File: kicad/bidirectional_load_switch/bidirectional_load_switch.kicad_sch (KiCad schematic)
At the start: 30 parts, among them J101 1017503, J102 Conn_01x02_Socket, J103 Conn_01x09_Socket, J104 Conn_01x02_Socket, J105 Conn_01x02_Socket, J106 Conn_01x02_Socket, J107 AVR-ISP-6, SW101 PTS526 SK15 SMTR2 LFS, U101 TMCS1101A3BQDRQ1, U102 TLV75733PDBVR, U103 ATTINY85-20SU

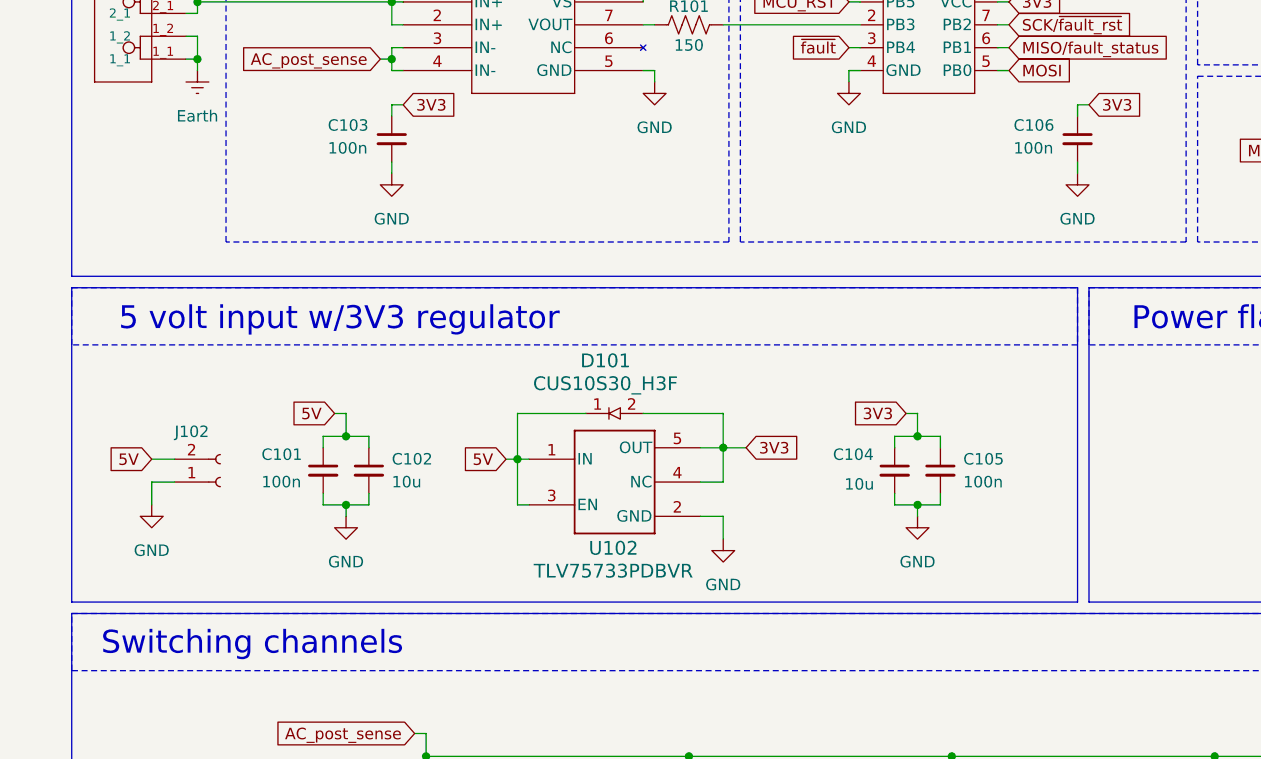
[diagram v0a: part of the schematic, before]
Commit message: ready for order
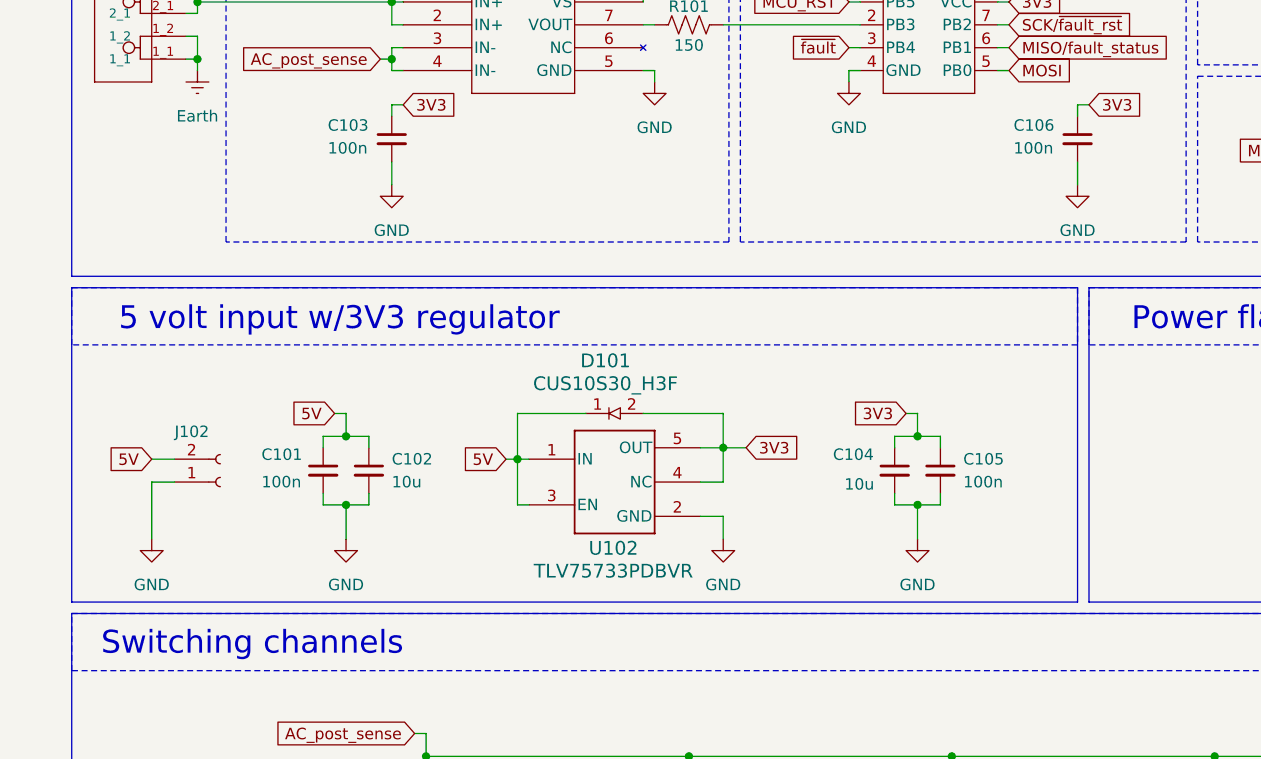
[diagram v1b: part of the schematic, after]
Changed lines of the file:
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@@
 	(wire
 		(pts
-			(xy 110.49 92.71) (xy 110.49 93.98)
+			(xy 110.49 92.71) (xy 110.49 96.52)
 		)
 		(stroke
@@
 	(wire
 		(pts
-			(xy 46.99 92.71) (xy 46.99 93.98)
+			(xy 46.99 92.71) (xy 46.99 96.52)
 		)
 		(stroke
@@
 	(wire
 		(pts
-			(xy 128.27 54.61) (xy 128.27 55.88)
+			(xy 128.27 54.61) (xy 128.27 57.15)
 		)
 		(stroke
@@
 	(wire
 		(pts
-			(xy 52.07 54.61) (xy 52.07 55.88)
+			(xy 52.07 54.61) (xy 52.07 57.15)
 		)
 		(stroke
@@
 	(wire
 		(pts
-			(xy 25.4 92.71) (xy 25.4 90.17)
+			(xy 25.4 96.52) (xy 25.4 90.17)
 		)
 		(stroke
@@
 	(symbol
 		(lib_id "power:GND")
-		(at 128.27 55.88 0)
+		(at 128.27 57.15 0)
 		(unit 1)
 		(exclude_from_sim no)
@@
 		(fields_autoplaced yes)
 		(property "Reference" "#PWR0111"
-			(at 128.27 62.23 0)
+			(at 128.27 63.5 0)
 			(effects
 				(font
@@
 		)
 		(property "Value" "GND"
-			(at 128.27 60.96 0)
+			(at 128.27 62.23 0)
 			(effects
 				(font
@@
 		)
 		(property "Footprint" ""
-			(at 128.27 55.88 0)
+			(at 128.27 57.15 0)
 			(effects
 				(font
@@
 		)
 		(property "Datasheet" ""
-			(at 128.27 55.88 0)
+			(at 128.27 57.15 0)
 			(effects
 				(font
@@
 		)
 		(property "Description" "Power symbol creates a global label with name \"GND\" , ground"
-			(at 128.27 55.88 0)
+			(at 128.27 57.15 0)
 			(effects
 				(font
@@
 	(symbol
 		(lib_id "power:GND")
-		(at 25.4 92.71 0)
+		(at 25.4 96.52 0)
 		(unit 1)
 		(exclude_from_sim no)
@@
 		(fields_autoplaced yes)
 		(property "Reference" "#PWR0101"
-			(at 25.4 99.06 0)
+			(at 25.4 102.87 0)
 			(effects
 				(font
@@
 		)
 		(property "Value" "GND"
-			(at 25.4 97.79 0)
+			(at 25.4 101.6 0)
 			(effects
 				(font
@@
 		)
 		(property "Footprint" ""
-			(at 25.4 92.71 0)
+			(at 25.4 96.52 0)
 			(effects
 				(font
@@
 		)
 		(property "Datasheet" ""
-			(at 25.4 92.71 0)
+			(at 25.4 96.52 0)
 			(effects
 				(font
@@
 		)
 		(property "Description" "Power symbol creates a global label with name \"GND\" , ground"
-			(at 25.4 92.71 0)
+			(at 25.4 96.52 0)
 			(effects
 				(font
@@
 	(symbol
 		(lib_id "power:GND")
-		(at 52.07 55.88 0)
+		(at 52.07 57.15 0)
 		(unit 1)
 		(exclude_from_sim no)
@@
 		(fields_autoplaced yes)
 		(property "Reference" "#PWR0105"
-			(at 52.07 62.23 0)
+			(at 52.07 63.5 0)
 			(effects
 				(font
@@
 		)
 		(property "Value" "GND"
-			(at 52.07 60.96 0)
+			(at 52.07 62.23 0)
 			(effects
 				(font
@@
 		)
 		(property "Footprint" ""
-			(at 52.07 55.88 0)
+			(at 52.07 57.15 0)
 			(effects
 				(font
@@
 		)
 		(property "Datasheet" ""
-			(at 52.07 55.88 0)
+			(at 52.07 57.15 0)
 			(effects
 				(font
@@
 		)
 		(property "Description" "Power symbol creates a global label with name \"GND\" , ground"
-			(at 52.07 55.88 0)
+			(at 52.07 57.15 0)
 			(effects
 				(font
@@
 	(symbol
 		(lib_id "power:GND")
-		(at 110.49 93.98 0)
+		(at 110.49 96.52 0)
 		(unit 1)
 		(exclude_from_sim no)
@@
 		(fields_autoplaced yes)
 		(property "Reference" "#PWR0110"
-			(at 110.49 100.33 0)
+			(at 110.49 102.87 0)
 			(effects
 				(font
@@
 		)
 		(property "Value" "GND"
-			(at 110.49 99.06 0)
+			(at 110.49 101.6 0)
 			(effects
 				(font
@@
 		)
 		(property "Footprint" ""
-			(at 110.49 93.98 0)
+			(at 110.49 96.52 0)
 			(effects
 				(font
@@
 		)
 		(property "Datasheet" ""
-			(at 110.49 93.98 0)
+			(at 110.49 96.52 0)
 			(effects
 				(font
@@
 		)
 		(property "Description" "Power symbol creates a global label with name \"GND\" , ground"
-			(at 110.49 93.98 0)
+			(at 110.49 96.52 0)
 			(effects
 				(font
@@
 	(symbol
 		(lib_id "power:GND")
-		(at 46.99 93.98 0)
+		(at 46.99 96.52 0)
 		(unit 1)
 		(exclude_from_sim no)
@@
 		(fields_autoplaced yes)
 		(property "Reference" "#PWR0104"
-			(at 46.99 100.33 0)
+			(at 46.99 102.87 0)
 			(effects
 				(font
@@
 		)
 		(property "Value" "GND"
-			(at 46.99 99.06 0)
+			(at 46.99 101.6 0)
 			(effects
 				(font
@@
 		)
 		(property "Footprint" ""
-			(at 46.99 93.98 0)
+			(at 46.99 96.52 0)
 			(effects
 				(font
@@
 		)
 		(property "Datasheet" ""
-			(at 46.99 93.98 0)
+			(at 46.99 96.52 0)
 			(effects
 				(font
@@
 		)
 		(property "Description" "Power symbol creates a global label with name \"GND\" , ground"
-			(at 46.99 93.98 0)
+			(at 46.99 96.52 0)
 			(effects
 				(font
